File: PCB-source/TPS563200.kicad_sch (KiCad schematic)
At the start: 0 parts

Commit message: Finish component and diffpair placement
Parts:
- added C17: 100nF, PCM_JLCPCB:C_0402, symbol PCM_JLCPCB-Capacitors:0402,100nF,(2)
- added C18, C19, C20: 22uF, PCM_JLCPCB:C_0805, symbol PCM_JLCPCB-Capacitors:0805,22uF
- added D2: Red, PCM_JLCPCB:D_0603, symbol PCM_JLCPCB-Diodes:LED,0603,Red
- added JP301: SolderJumper_2_Bridged, Jumper:SolderJumper-2_P1.3mm_Open_TrianglePad1.0x1.5mm, symbol Jumper:SolderJumper_2_Bridged
- added L301: 3.3uH, Inductor_SMD:L_Changjiang_FXL0420, symbol Device:L
- added R11: 33.2kΩ, PCM_JLCPCB:R_0402, symbol PCM_JLCPCB-Resistors:0402,10kΩ
- added R13: 680Ω, PCM_JLCPCB:R_0402, symbol PCM_JLCPCB-Resistors:0402,680Ω
- added R307: 10kΩ, PCM_JLCPCB:R_0402, symbol PCM_JLCPCB-Resistors:0402,10kΩ
- added TP302: TestPoint, TestPoint:TestPoint_Pad_D1.0mm, symbol Connector:TestPoint
- added U301: TPS563200, Package_TO_SOT_SMD:SOT-23-6, symbol Regulator_Switching:TPS563200
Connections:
- new net: D2.1, R13.1
- new net +3V3_UNPROTEC: C18.1, C20.1, D2.2, JP301.1 (A), L301.2, R11.1
- new net FB_3V3: R11.2, R307.1, U301.4 (VFB)
- new net GND: C18.2, C19.2, C20.2, R13.2, R307.2, U301.1 (GND)
- new net SW_3V3: C17.1, L301.1, U301.2 (SW)
- new net VBST_3V3: C17.2, U301.6 (VBST)
- new net VOUT: JP301.2 (B), TP302.1
- new net Vin: C19.1, U301.3 (VIN), U301.5 (EN)
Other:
- note added: "V_{OUT} = 0.765*(1+33k2/10k) = 3.3V"
- note added: "V_{OUT} = 0.765*(1+R302/R307)"

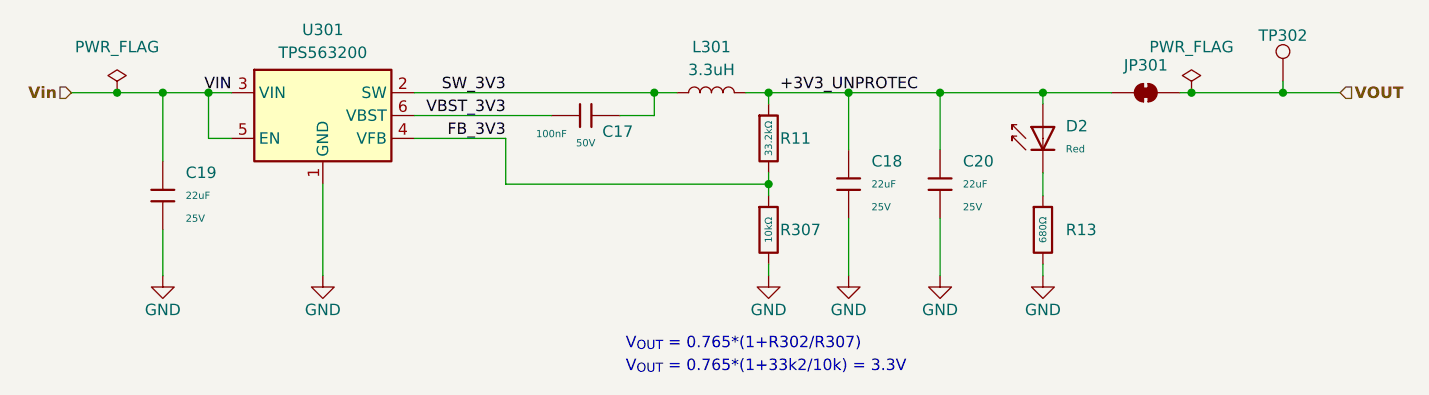
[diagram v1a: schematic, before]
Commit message: pinout start
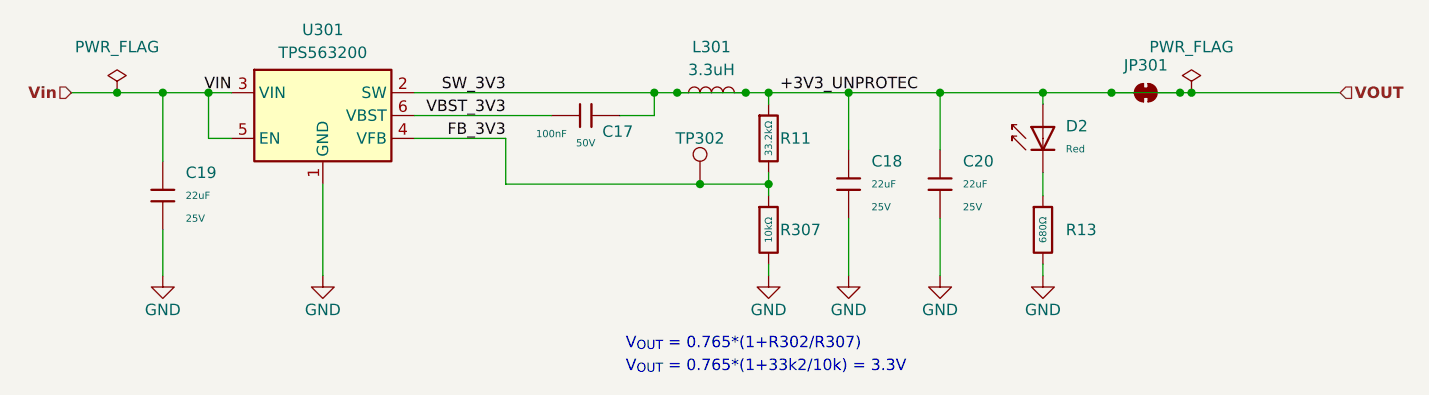
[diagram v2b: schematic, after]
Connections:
- net +3V3_UNPROTEC is gone; now on net VOUT: C18.1, C20.1, D2.2, JP301.1 (A), L301.2, R11.1
- net SW_3V3 is gone; now on net VOUT: C17.1, L301.1, U301.2 (SW)
- net FB_3V3: now also TP302.1
- net VOUT: no longer TP302.1
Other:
- moved on the sheet: TP302
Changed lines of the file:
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@@
 	)
 	(junction
-		(at 208.28 90.17)
+		(at 143.51 100.33)
+		(diameter 0)
+		(color 0 0 0 0)
+	)
+	(junction
+		(at 148.59 90.17)
 		(diameter 0)
 		(color 0 0 0 0)
@@
 	)
 	(junction
+		(at 189.23 90.17)
+		(diameter 0)
+		(color 0 0 0 0)
+	)
+	(junction
 		(at 160.02 90.17)
 		(diameter 0)
@@
 	)
 	(junction
+		(at 196.85 90.17)
+		(diameter 0)
+		(color 0 0 0 0)
+	)
+	(junction
 		(at 151.13 100.33)
+		(diameter 0)
+		(color 0 0 0 0)
+	)
+	(junction
+		(at 140.97 90.17)
 		(diameter 0)
 		(color 0 0 0 0)
@@
 	(wire
 		(pts
+			(xy 181.61 90.17) (xy 189.23 90.17)
+		)
+		(stroke
+			(width 0)
+			(type default)
+		)
+	)
+	(wire
+		(pts
 			(xy 83.82 97.79) (xy 83.82 90.17)
 		)
@@
 	(wire
 		(pts
-			(xy 208.28 88.9) (xy 208.28 90.17)
-		)
-		(stroke
-			(width 0)
-			(type default)
-		)
-	)
-	(wire
-		(pts
 			(xy 88.9 95.25) (xy 91.44 95.25)
 		)
@@
 	(wire
 		(pts
+			(xy 189.23 90.17) (xy 196.85 90.17)
+		)
+		(stroke
+			(width 0)
+			(type default)
+		)
+	)
+	(wire
+		(pts
 			(xy 151.13 90.17) (xy 160.02 90.17)
 		)
@@
 	(wire
 		(pts
+			(xy 140.97 90.17) (xy 148.59 90.17)
+		)
+		(stroke
+			(width 0)
+			(type default)
+		)
+	)
+	(wire
+		(pts
 			(xy 170.18 90.17) (xy 181.61 90.17)
 		)
@@
 	(wire
 		(pts
+			(xy 198.12 90.17) (xy 214.63 90.17)
+		)
+		(stroke
+			(width 0)
+			(type default)
+		)
+	)
+	(wire
+		(pts
 			(xy 181.61 90.17) (xy 181.61 91.44)
 		)
@@
 	(wire
 		(pts
-			(xy 121.92 100.33) (xy 151.13 100.33)
+			(xy 121.92 100.33) (xy 143.51 100.33)
+		)
+		(stroke
+			(width 0)
+			(type default)
+		)
+	)
+	(wire
+		(pts
+			(xy 143.51 100.33) (xy 151.13 100.33)
 		)
 		(stroke
@@
 	(wire
 		(pts
-			(xy 198.12 90.17) (xy 208.28 90.17)
-		)
-		(stroke
-			(width 0)
-			(type default)
-		)
-	)
-	(wire
-		(pts
 			(xy 78.74 90.17) (xy 83.82 90.17)
 		)
@@
 	(wire
 		(pts
-			(xy 189.23 90.17) (xy 181.61 90.17)
-		)
-		(stroke
-			(width 0)
-			(type default)
-		)
-	)
-	(wire
-		(pts
 			(xy 151.13 91.44) (xy 151.13 90.17)
-		)
-		(stroke
-			(width 0)
-			(type default)
-		)
-	)
-	(wire
-		(pts
-			(xy 208.28 90.17) (xy 214.63 90.17)
 		)
 		(stroke
@@
 	(symbol
 		(lib_id "Connector:TestPoint")
-		(at 208.28 88.9 0)
+		(at 143.51 100.33 0)
 		(unit 1)
 		(exclude_from_sim no)
@@
 		(dnp no)
 		(property "Reference" "TP302"
-			(at 208.28 83.82 0)
+			(at 143.51 95.25 0)
 			(effects
 				(font
@@
 		)
 		(property "Value" "TestPoint"
-			(at 210.82 86.868 0)
+			(at 146.05 98.298 0)
 			(effects
 				(font
@@
 		)
 		(property "Footprint" "TestPoint:TestPoint_Pad_D1.0mm"
-			(at 213.36 88.9 0)
+			(at 148.59 100.33 0)
 			(effects
 				(font
@@
 		)
 		(property "Datasheet" "~"
-			(at 213.36 88.9 0)
+			(at 148.59 100.33 0)
 			(effects
 				(font
@@
 		)
 		(property "Description" "test point"
-			(at 208.28 88.9 0)
-			(effects
-				(font
+			(at 143.51 100.33 0)
+			(effects
+				(font
